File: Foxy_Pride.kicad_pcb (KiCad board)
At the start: 2 copper layers, 89.3 x 67.9 mm, 33 parts, among them U1 TLC555CDR, U2 74HC4017D

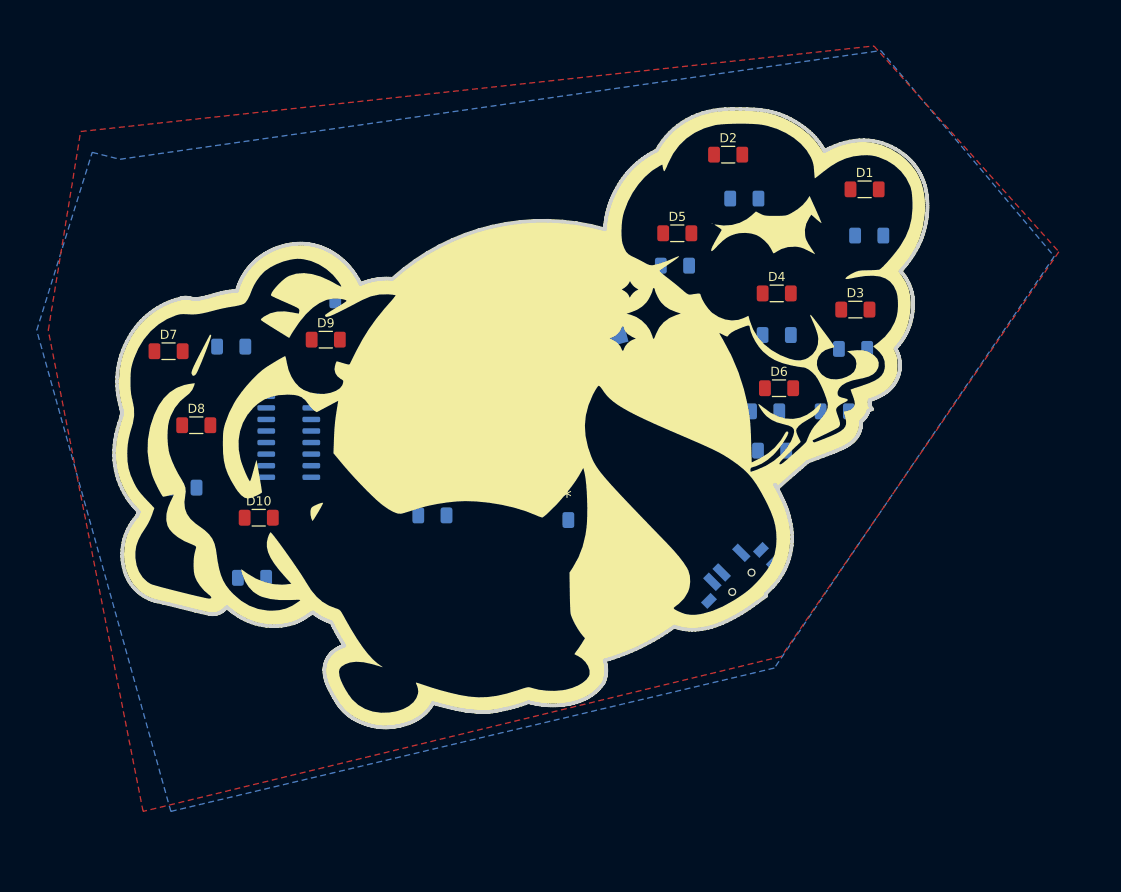
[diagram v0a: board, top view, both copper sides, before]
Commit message: PCB Layout
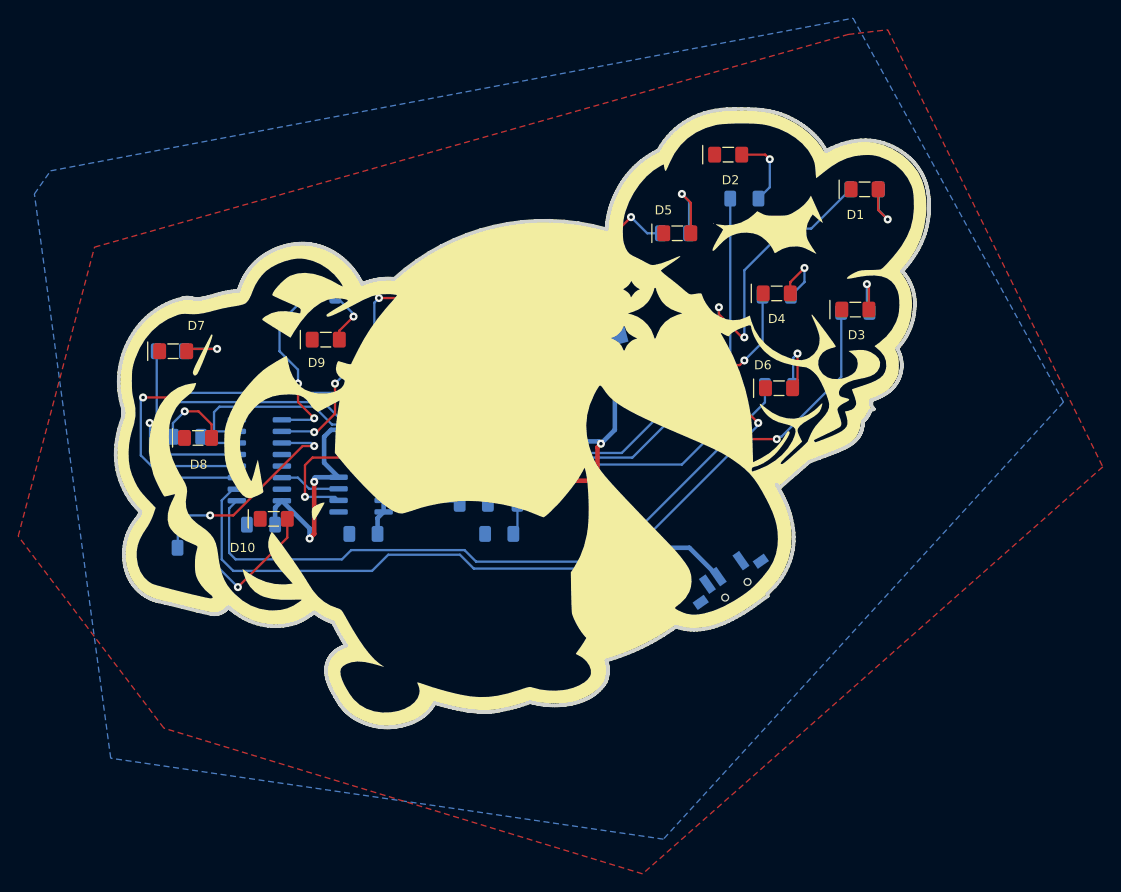
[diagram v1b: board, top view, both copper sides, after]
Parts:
- added G***: LOGO, Alpenglow:Alpenglow_Logo_Horiz_8mm, B.Cu at (87.9, 74.2)
- D1, D10, D2, D3, D4, D5, D6, D7, D8, D9: footprint Resistor_SMD:R_1206_3216Metric_Pad1.30x1.75mm_HandSolder -> Alpenglow:LED_1206+
- U1: footprint Package_SO:SOIC-8_3.9x4.9mm_P1.27mm -> Alpenglow:SO-8
- U2: footprint Package_SO:SOIC-16_3.9x9.9mm_P1.27mm -> Alpenglow:SO-16
- moved C1 31.3 mm to (68.6, 81.3)
- moved R1 27.8 mm to (65.8, 78.0), turned to 0 degrees
- moved R2 27.6 mm to (72.1, 78.0)
- moved C3 25.4 mm to (53.4, 72.4)
- moved C4 18.8 mm to (42.4, 80.3)
- moved C2 18.2 mm to (53.7, 81.3)
- moved R12 7.41 mm to (34.8, 82.8)
- moved R8 6.73 mm to (99.3, 65.0)
- moved R9 6.65 mm to (32.5, 61.2)
- moved U1 6.45 mm to (53.4, 77.0), turned to 0 degrees
- moved R10 5.61 mm to (34.3, 70.6), turned to 0 degrees
- moved R3 5.11 mm to (108.7, 43.4)
- moved R6 4.32 mm to (99.1, 55.1)
- moved U2 4.14 mm to (42.2, 73.2)
- moved R5 4.07 mm to (107.7, 56.9)
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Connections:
- net Net-(U1-Pad3) renamed /CLOCK
- BT1 pad 1: Net-(BT1-Pad1) -> +3V
- S1 pad 1: Net-(BT1-Pad1) -> GND
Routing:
- net +3V: track 0.00 -> 147.2 mm, vias 0 -> 5
- net Net-(R3-Pad2): track 0.00 -> 121.3 mm, vias 0 -> 4
- net Net-(R5-Pad2): track 0.00 -> 105.2 mm, vias 0 -> 4
- net Net-(R4-Pad2): track 0.00 -> 102.6 mm, vias 0 -> 2
- net Net-(R6-Pad2): track 0.00 -> 82.7 mm, vias 0 -> 2
- net Net-(R8-Pad2): track 0.00 -> 75.2 mm
- net Net-(R7-Pad2): track 0.00 -> 56.8 mm, vias 0 -> 4
- net Net-(R1-Pad2): track 0.00 -> 46.7 mm, vias 0 -> 4
- net Net-(R12-Pad2): track 0.00 -> 24.8 mm, vias 0 -> 2
- net Net-(R11-Pad2): track 0.00 -> 19.9 mm, vias 0 -> 2
- net Net-(R9-Pad2): track 0.00 -> 19.6 mm
- net Net-(D10-Pad2): track 0.00 -> 15.5 mm, vias 0 -> 1
- net Net-(D5-Pad2): track 0.00 -> 9.37 mm, vias 0 -> 1
- net Net-(D8-Pad2): track 0.00 -> 8.37 mm, vias 0 -> 1
- net Net-(D2-Pad2): track 0.00 -> 8.13 mm, vias 0 -> 1
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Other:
- board text added: "Foxy Pride"
- board text added: "OFF"
- board text added: "ON"
